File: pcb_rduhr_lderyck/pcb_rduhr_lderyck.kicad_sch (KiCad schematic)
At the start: 56 parts, among them J1 Conn_ARM_JTAG_SWD_10, J2 Résistance chauffante, J3 Conn_15_-15, J4 Conn_1.8, J5 Probe_15, J6 Probe_-15, J7 RX_TX, J8 RF, Q1 NMOS, Q2 NMOS, SW1 SW_DPDT_x2, U1 STM32F030F4Px, U2 AP7333, U3 MCP9700Ax-ETT, U4 MIC5271, Y1 Crystal_Small

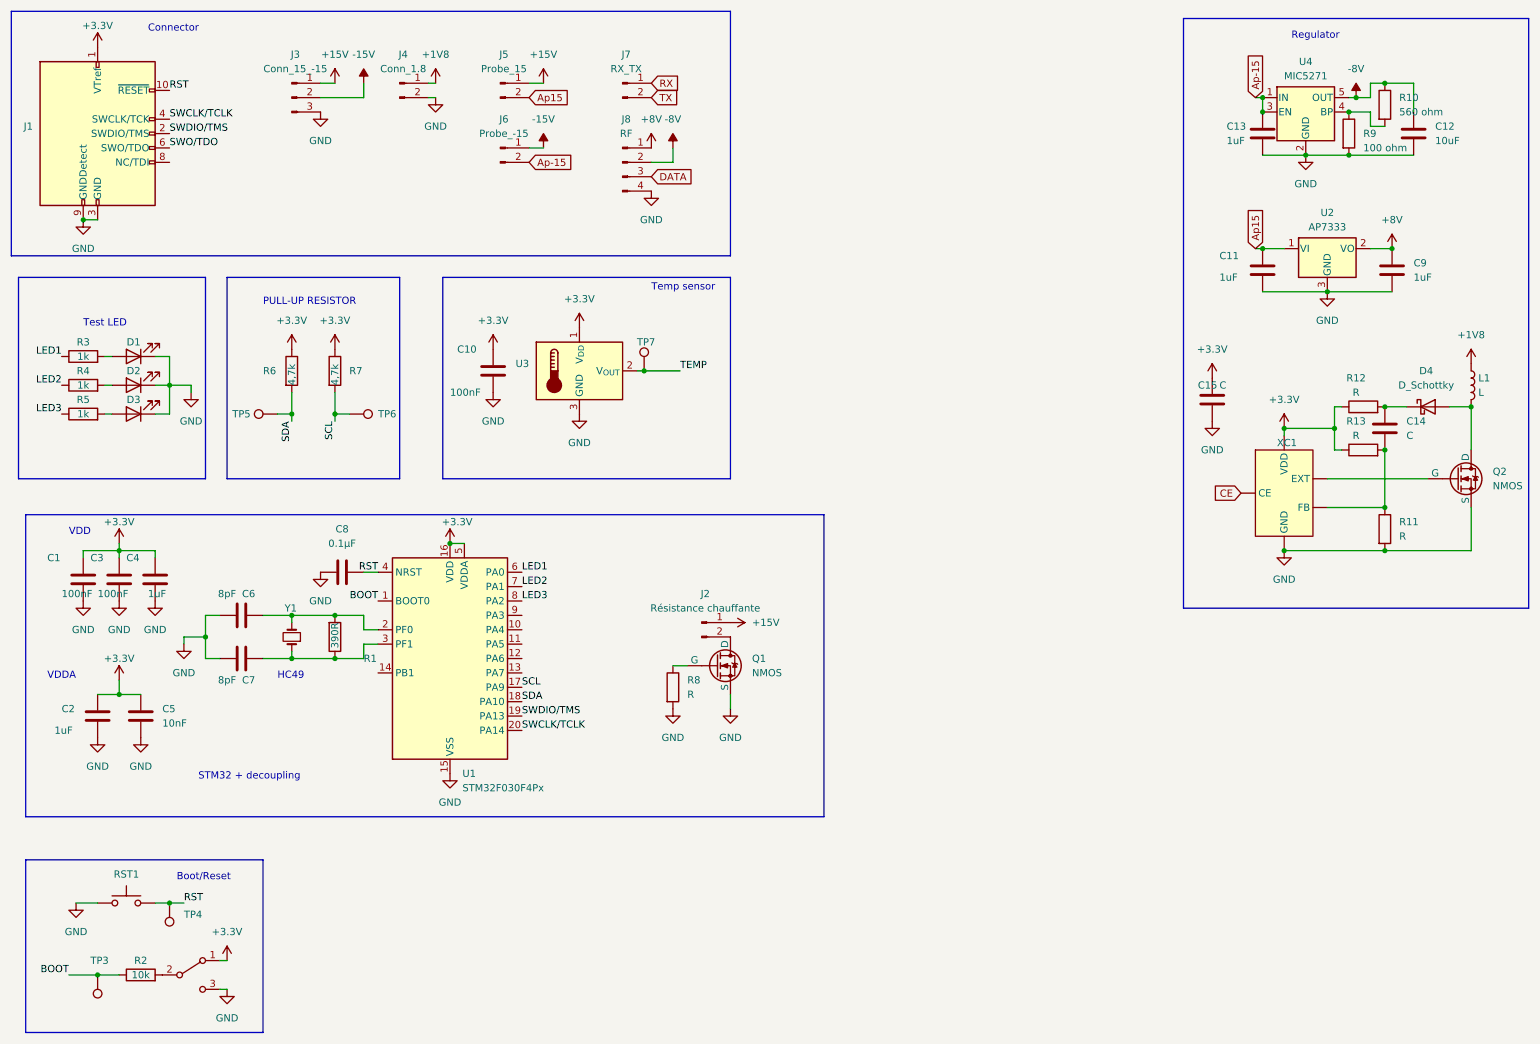
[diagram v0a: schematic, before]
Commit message: Update PCB 1
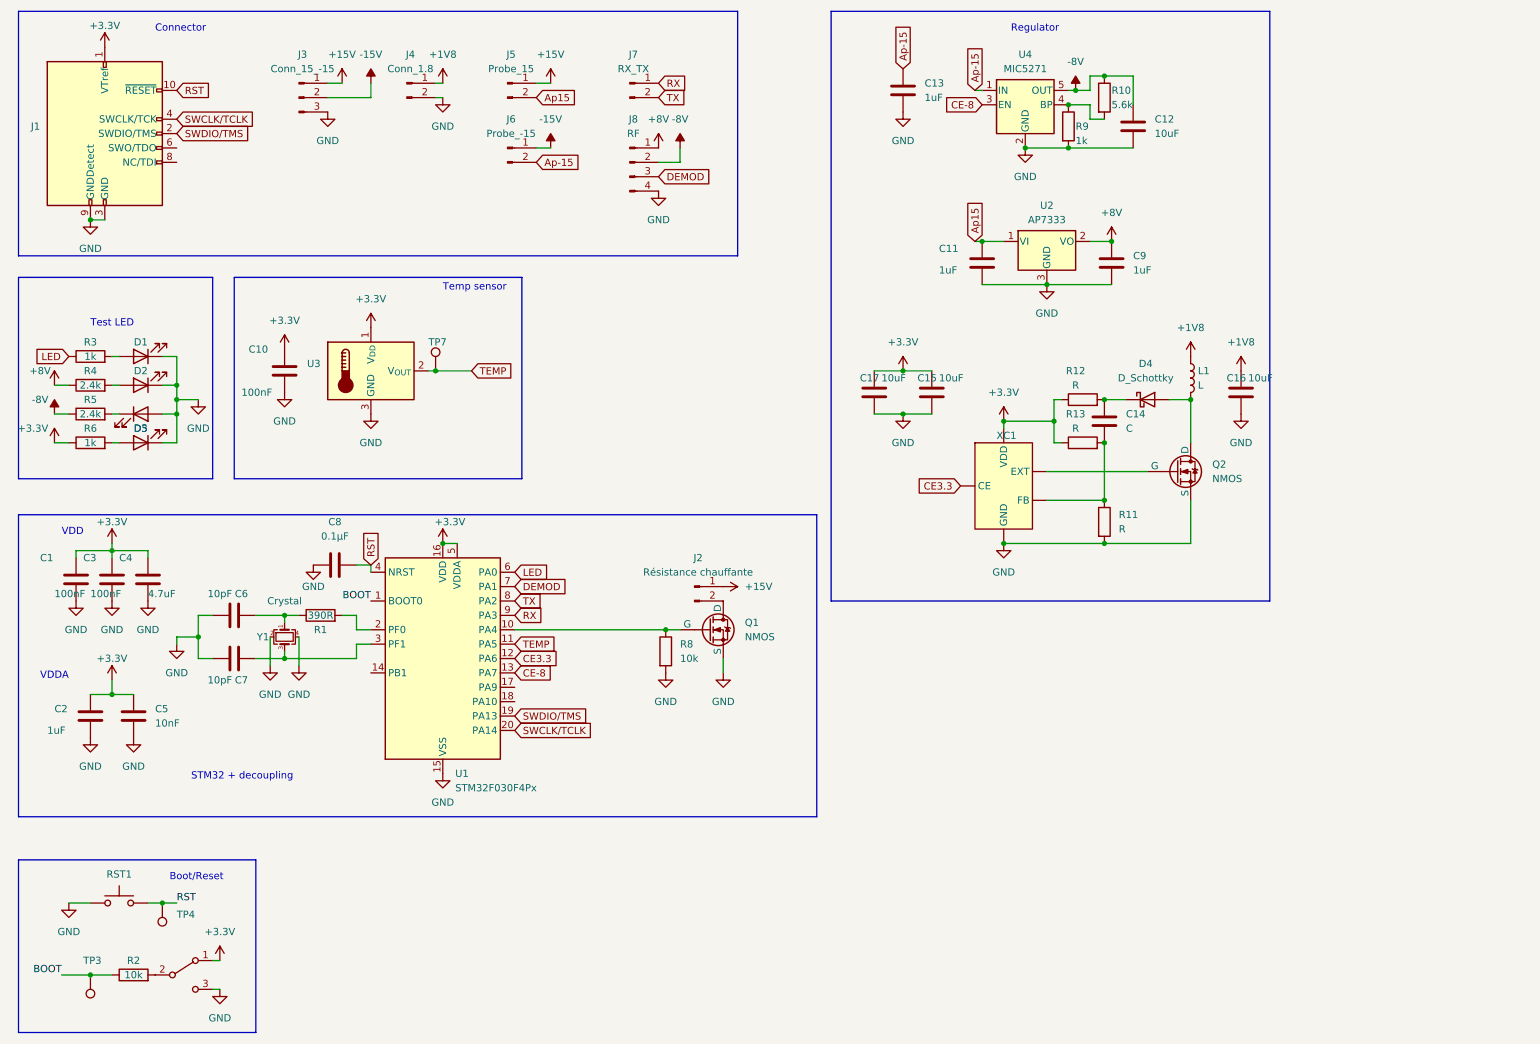
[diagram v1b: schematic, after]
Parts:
- removed R7: 4,7k, Resistor_SMD:R_0603_1608Metric_Pad0.98x0.95mm_HandSolder, symbol Device:R
- removed TP5, TP6: TestPoint, TestPoint:TestPoint_Pad_D1.5mm, symbol Connector:TestPoint
- removed Y1: Crystal_Small, Crystal:Crystal_SMD_HC49-SD_HandSoldering, symbol Device:Crystal_Small
- added C16, C17: 10uF, Capacitor_SMD:C_0603_1608Metric_Pad1.08x0.95mm_HandSolder, symbol Device:C
- added D5: LED, Diode_SMD:D_0603_1608Metric_Pad1.05x0.95mm_HandSolder, symbol Device:LED
- added Y1: Crystal, symbol Device:Crystal_GND24_Small
- C11, C12, C13, C14, C9: footprint (none) -> Capacitor_SMD:C_0603_1608Metric_Pad1.08x0.95mm_HandSolder
- C15: value C -> 10uF; footprint (none) -> Capacitor_SMD:C_0603_1608Metric_Pad1.08x0.95mm_HandSolder
- C4: value 1uF -> 4.7uF
- C6, C7: value 8pF -> 10pF
- R1: footprint Resistor_SMD:R_0603_1608Metric_Pad0.98x0.95mm_HandSolder -> (none)
- R10: value 560 ohm -> 5.6k
- R4, R5: value 1k -> 2.4k
- R6: value 4,7k -> 1k
- R8: value R -> 10k
- R9: value 100 ohm -> 1k
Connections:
- net CE is gone; now on net GND: XC1. (VDD)
- net +1V8: now also C16.1
- net +3.3V: now also C17.1
- net +8V: now also R4.1
- net -8V: now also R5.1
- net Ap-15: now also C13.1; no longer C13.2, U4.3 (EN)
- net GND: now also C13.2, D3.2 (A), C16.2, C17.2, D5.1 (K), Y1.2, Y1.4; no longer C13.1, D3.1 (K)
- net RX: now also U1.9 (PA3)
- net TEMP: now also U1.11 (PA5)
- net TX: now also U1.8 (PA2)
- net at R1.2, U1.2 (PF0): no longer C6.1
- net at R5.2: now also D3.1 (K); no longer D3.2 (A)
- net at C7.1, U1.3 (PF1): now also Y1.3; no longer R1.1
- net at Q1.2 (G), R8.1: now also U1.10 (PA4)
- net CE3.3: now reaches U1.12 (PA6)
- net CE3.3: now also XC1. (VDD)
- net CE-8: now reaches U1.13 (PA7)
- net CE-8: now also U4.3 (EN)
- net DATA renamed DEMOD
- net DEMOD: now also U1.7 (PA1)
- net LED1 renamed LED
- removed net LED2: R4.1, U1.7 (PA1)
- removed net LED3: R5.1, U1.8 (PA2)
- net SCL: no longer names the net of U1.17 (PA9)
- net SDA: no longer names the net of R6.2
- net SDA: now also D5.2 (A); no longer U1.18 (PA10)
- net SWO/TDO: no longer names the net of J1.6 (SWO/TDO)
- new net: C6.1, R1.1, Y1.1
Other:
- note removed: "HC49"
- note removed: "PULL-UP RESISTOR"
- moved on the sheet: C1, C10, C11, C12, C14, C15, C2, C3, C4, C5, C6, C7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
